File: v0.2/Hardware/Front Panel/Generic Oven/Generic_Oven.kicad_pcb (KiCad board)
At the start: 2 copper layers, 47 x 70 mm, 0 parts

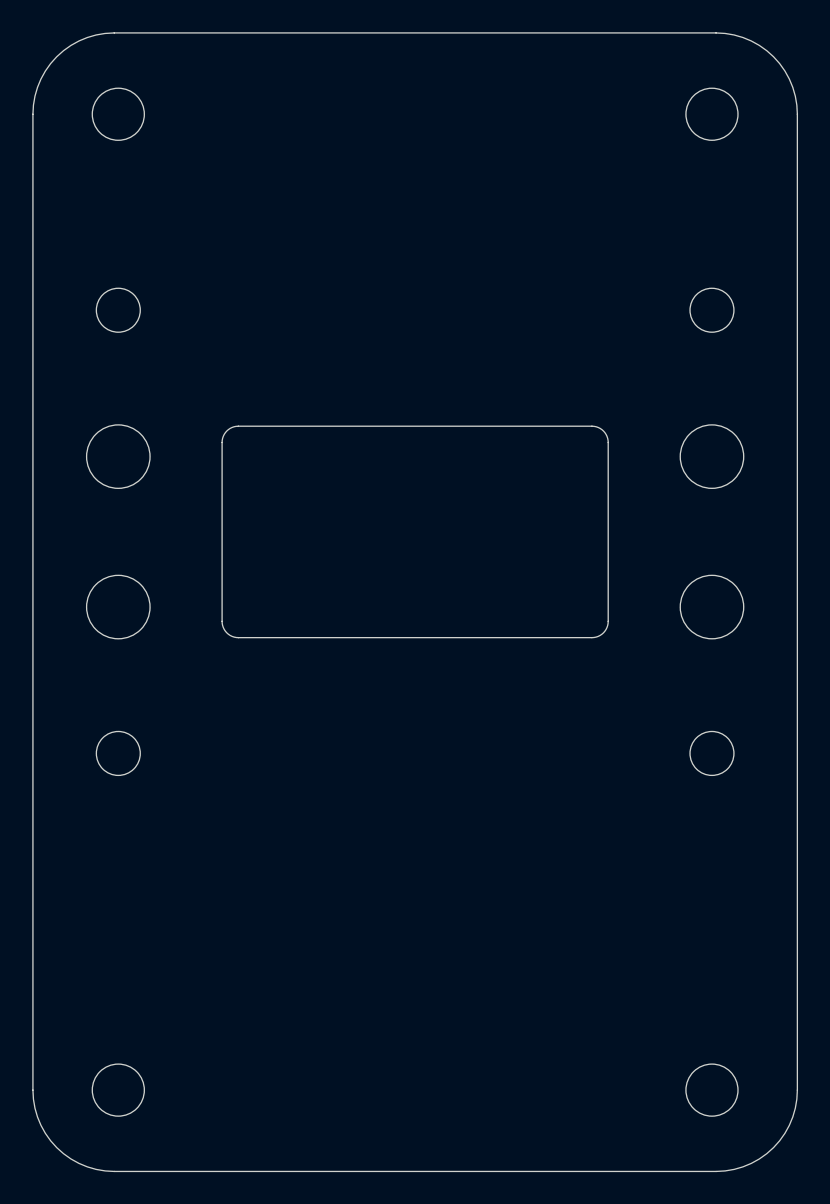
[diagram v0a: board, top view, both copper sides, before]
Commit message: v0.2: Finished PCBs
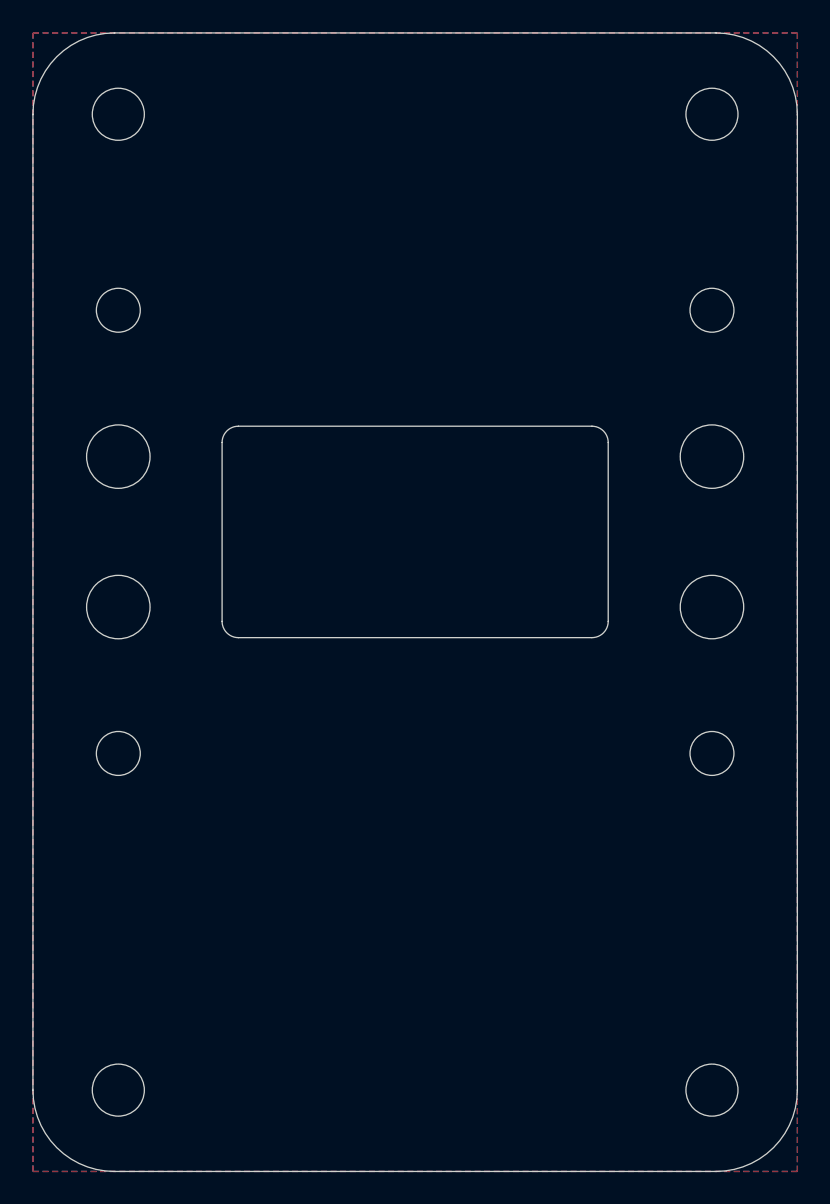
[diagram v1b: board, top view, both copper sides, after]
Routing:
- added copper zone on B.Cu, net (none)
- added copper zone on F.Cu, net (none)
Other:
- board text added: "BACK"
- board text added: "LUNA Embedded"
- board text added: "OK"
- board text added: "Reflow Controller"
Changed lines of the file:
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@@
-(kicad_pcb (version 20171130) (host pcbnew 5.1.9)
+(kicad_pcb (version 20171130) (host pcbnew 5.1.10)
   (general
     (thickness 1.6)
-    (drawings 37)
+    (drawings 43)
     (tracks 0)
     (zones 0)
@@
     (46 B.CrtYd user hide)
     (47 F.CrtYd user)
-    (48 B.Fab user)
+    (48 B.Fab user hide)
     (49 F.Fab user)
   )
@@
     (last_trace_width 0.25)
     (trace_clearance 0.2)
-    (zone_clearance 0.508)
+    (zone_clearance 0.2)
     (zone_45_only no)
     (trace_min 0.2)
@@
       (outputformat 1)
       (mirror false)
-      (drillshape 1)
+      (drillshape 0)
       (scaleselection 1)
-      (outputdirectory ""))
+      (outputdirectory "Gerbers/"))
   )
   (net 0 "")
@@
     (uvia_dia 0.3)
     (uvia_drill 0.1)
+  )
+  (gr_poly (pts (xy -19.7 3.55) (xy -16.8 3.55) (xy -18.25 5.05)) (layer F.Mask) (width 0.1))
+  (gr_poly (pts (xy -16.8 -12.2) (xy -19.7 -12.2) (xy -18.25 -13.7)) (layer F.Mask) (width 0.1))
+  (gr_text BACK (at 18.25 4.3) (layer F.Mask)
+    (effects (font (size 1.25 1.25) (thickness 0.25) italic))
+  )
+  (gr_text OK (at 18.25 -12.95) (layer F.Mask)
+    (effects (font (size 1.25 1.25) (thickness 0.25) italic))
+  )
+  (gr_text "LUNA Embedded" (at 0 30) (layer F.Mask)
+    (effects (font (size 1.5 1.5) (thickness 0.35) italic))
+  )
+  (gr_text "Reflow Controller" (at 0 -30) (layer F.Mask)
+    (effects (font (size 2 2) (thickness 0.45)))
   )
   (gr_circle (center 18.25 30) (end 19.85 30) (layer Edge.Cuts) (width 0.05))
@@
   (gr_circle (center 18.24 -8.95) (end 20.19 -8.95) (layer B.Fab) (width 0.05))
   (gr_circle (center 183.4 90.7) (end 182.1 89.1) (layer Dwgs.User) (width 0.15))
+  (zone (net 0) (net_name "") (layer F.Cu) (hatch edge 0.508)
+    (connect_pads yes (clearance 0.2))
+    (min_thickness 0.2)
+    (fill yes (arc_segments 32) (thermal_gap 0.2) (thermal_bridge_width 0.3))
+    (polygon
+      (pts
+        (xy 23.5 -35) (xy 23.5 35) (xy -23.5 35) (xy -23.5 -35)
+      )
+    )
+  )
+  (zone (net 0) (net_name "") (layer B.Cu) (hatch edge 0.508)
+    (connect_pads yes (clearance 0.2))
+    (min_thickness 0.2)
+    (fill yes (arc_segments 32) (thermal_gap 0.2) (thermal_bridge_width 0.3))
+    (polygon
+      (pts
+        (xy 23.5 -35) (xy 23.5 35) (xy -23.5 35) (xy -23.5 -35)
+      )
+    )
+  )
 )
